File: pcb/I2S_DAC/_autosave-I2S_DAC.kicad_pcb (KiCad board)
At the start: 2 copper layers, 35 parts, among them J1 AudioPlug3, J2 Conn_01x06, J3 Conn_01x09, U1 MIC5225-3.3YM5, U2 UDA1334ATS

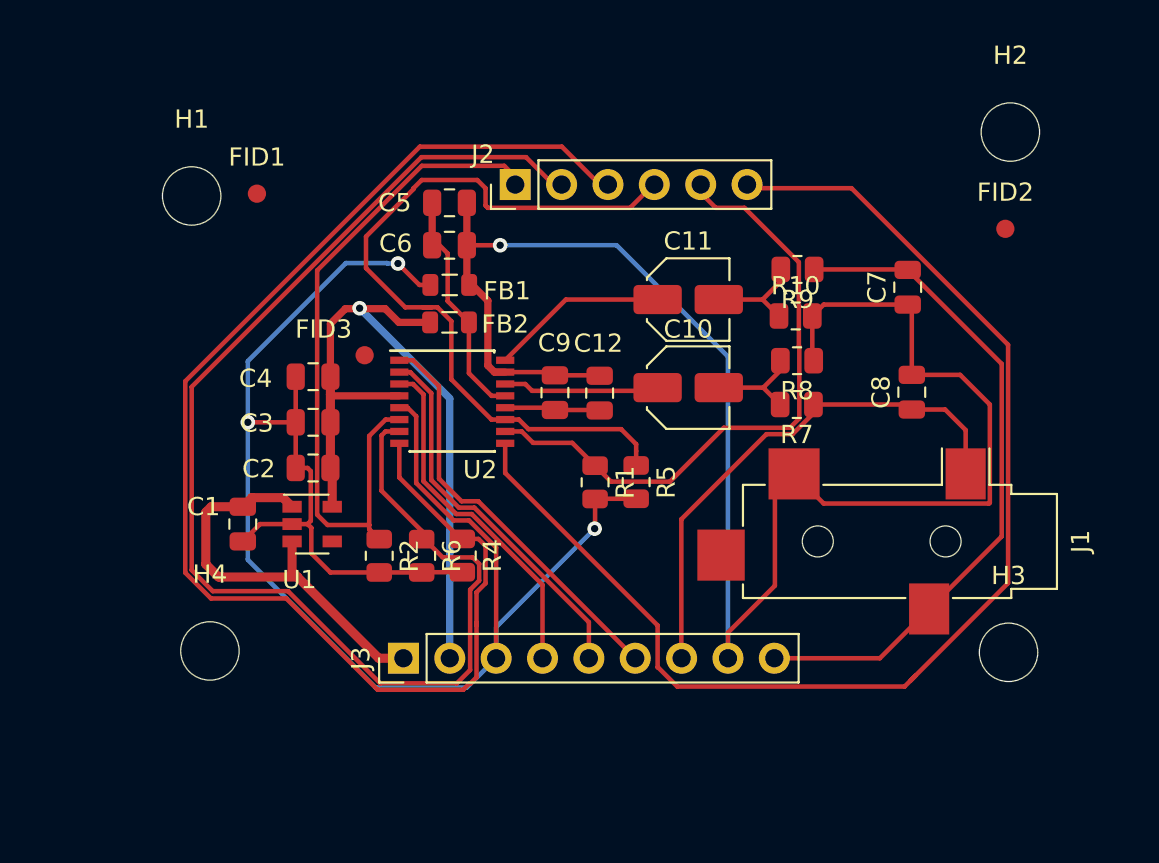
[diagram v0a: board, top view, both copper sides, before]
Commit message: Archivos finales presentacion 14-10-2021
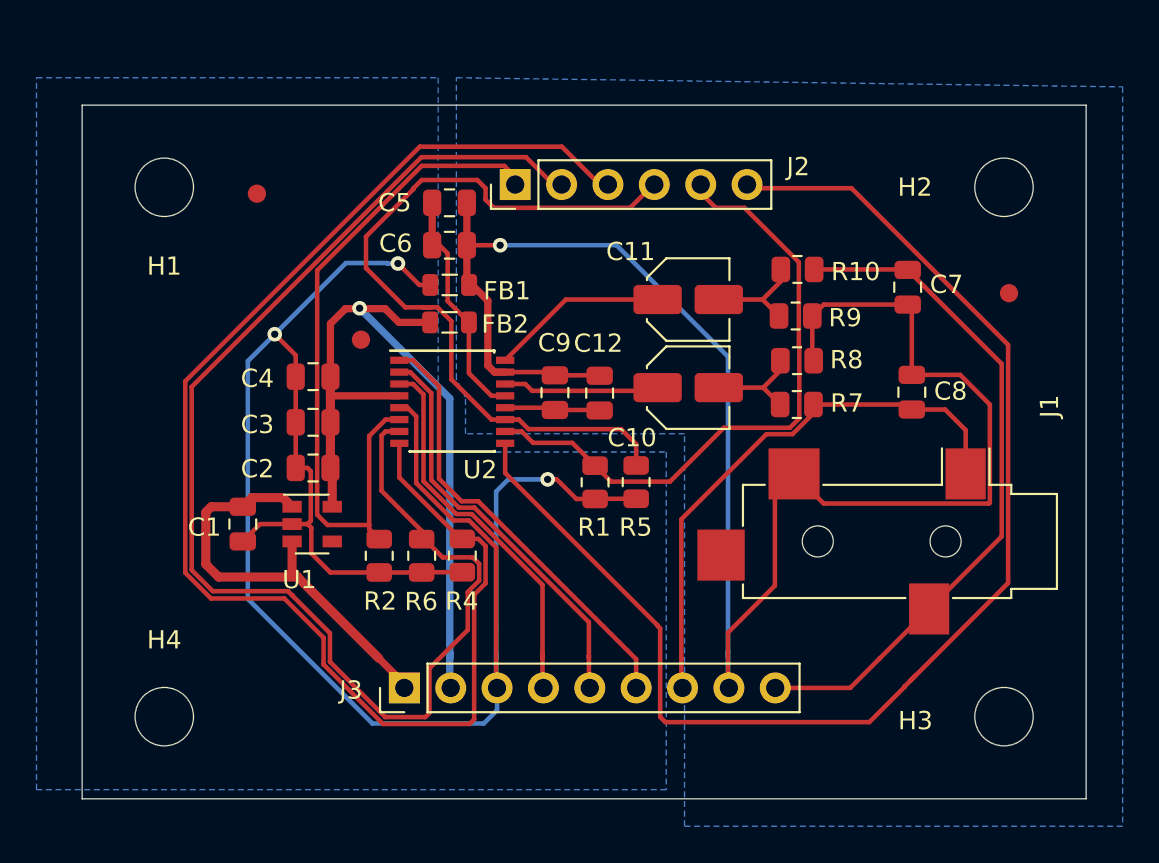
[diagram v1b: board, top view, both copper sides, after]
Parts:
- moved H4 4.38 mm to (47.5, 123.5)
- moved H3 3.53 mm to (93.5, 123.5)
- moved FID2 3.53 mm to (93.8, 100.3)
- moved H2 3.05 mm to (93.5, 94.5)
- moved J3 1.63 mm to (60.6, 121.9)
- moved H1 1.57 mm to (47.5, 94.5)
- moved FID3 0.87 mm to (58.3, 102.8)
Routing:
- net GNDD: track 96.5 -> 107.5 mm
- net GNDA: track 94.8 -> 98.4 mm
- net /MUTE: track 74.3 -> 77.8 mm
- net /CLKOUT: track 69.2 -> 72.4 mm
- net /SFOR_1: track 71.5 -> 74.0 mm
- net /DATA_IN: track 19.2 -> 21.2 mm
- net +3V3: track 41.2 -> 43.2 mm
- net /WS_IN: track 20.8 -> 22.6 mm
- net /OUT_L: track 29.1 -> 30.7 mm
- net /BCK_IN: track 22.7 -> 24.3 mm
- net VDD: track 23.1 -> 24.0 mm
- net /OUT_R: track 37.1 -> 37.7 mm
- added copper zone on B.Cu, net GNDA
- added copper zone on B.Cu, net GNDD
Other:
- board outline added: 55 x 38 mm
- board text added: "Especificaciones técnicas Grillas 0,5 mm - 0,25 mm Vias: 0,8 mm / 0,4 mm Margen global: 0,4 mm Margen local: 0,1 mm Pistas: 0,5 mm; 0,4 mm; 0,25 mm Dist. a borde: 0,5 mm Terminación: HASL ; Estaño-Plomo (Sn/Pb) Fabricante: Seed Studio Stack-up SIG F. Cu ____________________________ 1 oz Core 1,6 mm SIG B. Cu_____________________________ 1 oz"
